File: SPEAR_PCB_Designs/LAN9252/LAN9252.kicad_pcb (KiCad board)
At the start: 2 copper layers, 68 parts, among them J1 SM04B-GHS-TB, J3 SM04B-GHS-TB, SW2 SW_MEC_5E, T1 H1102NLT, T2 H1102NLT, U1 LAN9252_ML, U2 24FC512, Y1 25MHz

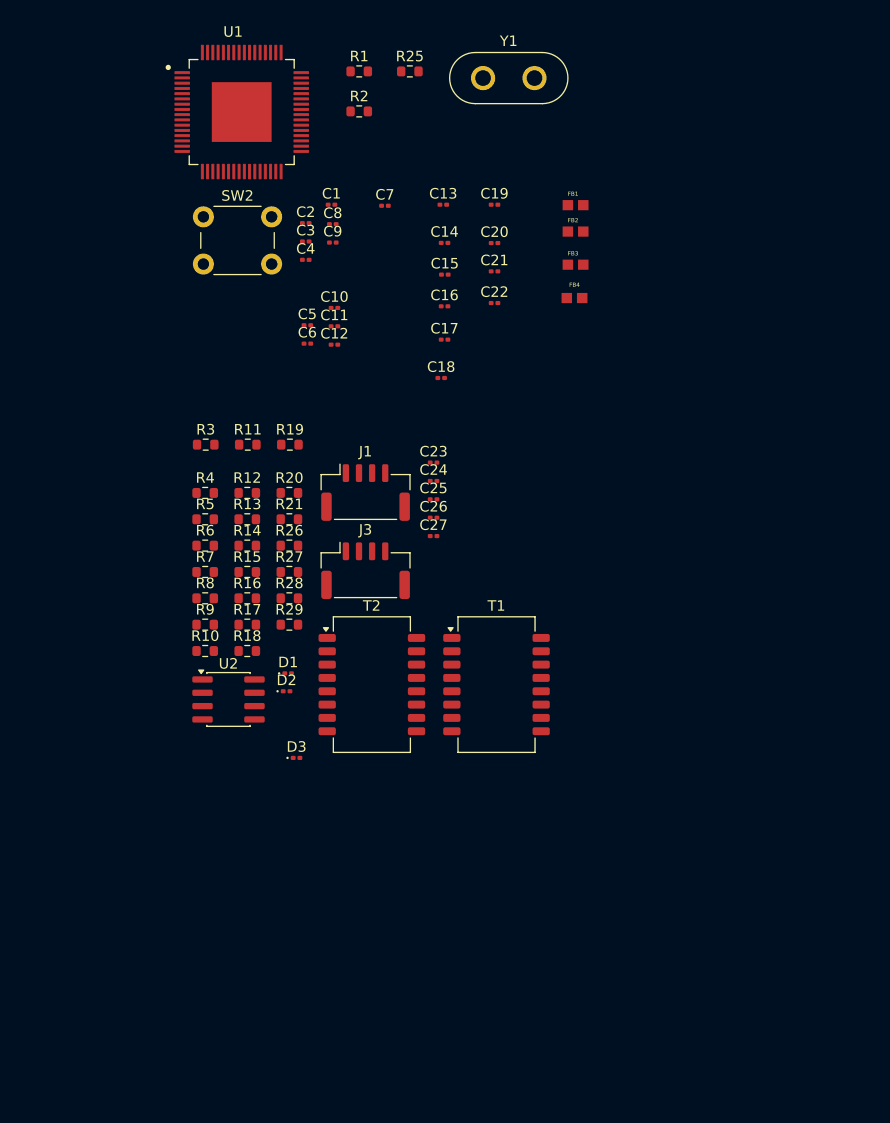
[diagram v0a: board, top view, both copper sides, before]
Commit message: Chris editted this.
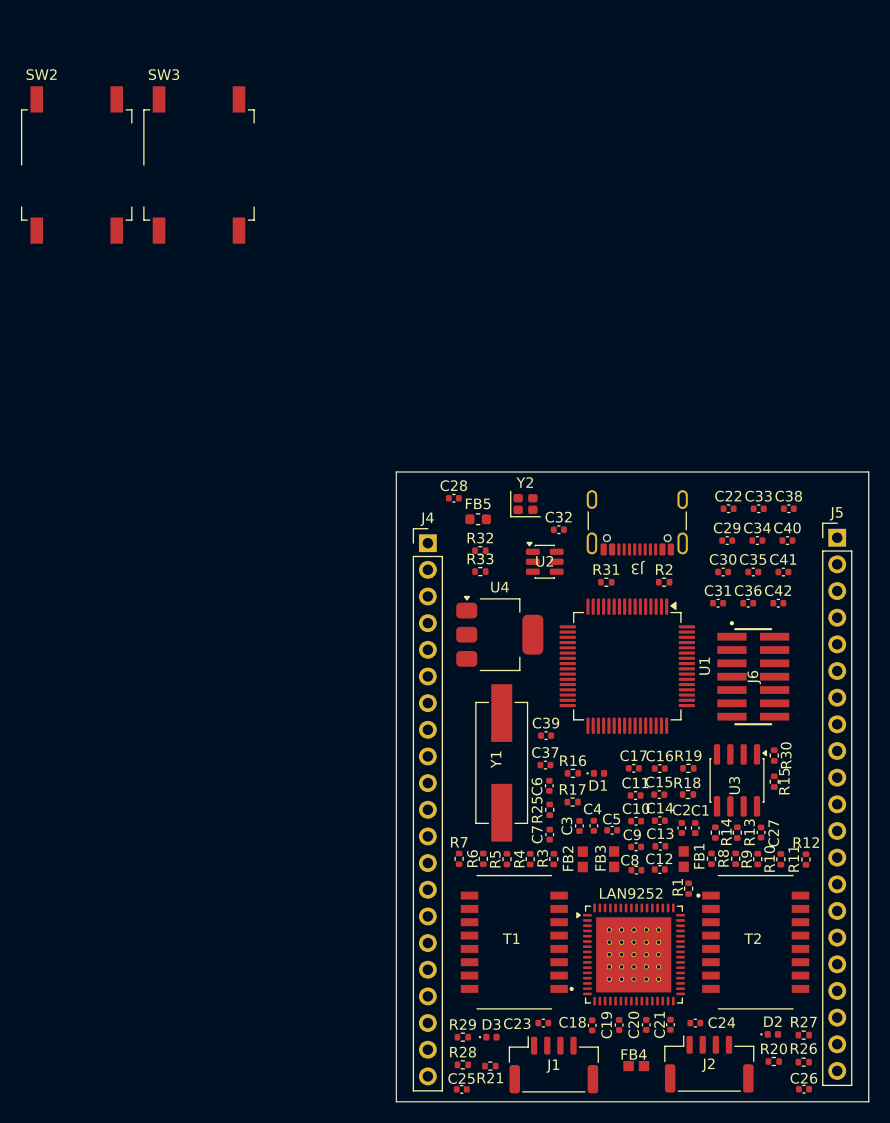
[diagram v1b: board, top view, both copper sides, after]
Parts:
- added C28: 10u, Capacitor_SMD:C_0402_1005Metric, F.Cu at (129.5, 90.8)
- added C29: 100n, Capacitor_SMD:C_0402_1005Metric, F.Cu at (155.5, 94.9)
- added C30: 10p, Capacitor_SMD:C_0402_1005Metric, F.Cu at (155.1, 97.9)
- added C31: 100n, Capacitor_SMD:C_0402_1005Metric, F.Cu at (154.7, 100.8)
- added C32: 100n, Capacitor_SMD:C_0402_1005Metric, F.Cu at (139.5, 93.8)
- added C33: 10p, Capacitor_SMD:C_0402_1005Metric, F.Cu at (158.5, 91.8)
- added C34: 100n, Capacitor_SMD:C_0402_1005Metric, F.Cu at (158.4, 94.9)
- added C35: 100n, Capacitor_SMD:C_0402_1005Metric, F.Cu at (158.0, 97.9)
- added C36: 2.2u, Capacitor_SMD:C_0402_1005Metric, F.Cu at (157.5, 100.8)
- added C37: 10u, Capacitor_SMD:C_0402_1005Metric, F.Cu at (138.2, 116.3)
- added C38: 100n, Capacitor_SMD:C_0402_1005Metric, F.Cu at (161.4, 91.8)
- added C39: 22u, Capacitor_SMD:C_0402_1005Metric, F.Cu at (138.3, 113.4)
- added C40: 10n, Capacitor_SMD:C_0402_1005Metric, F.Cu at (161.3, 94.9)
- added C41: 1u, Capacitor_SMD:C_0402_1005Metric, F.Cu at (160.9, 97.9)
- added C42: 1u, Capacitor_SMD:C_0402_1005Metric, F.Cu at (160.4, 100.8)
- added FB5: 120R, Inductor_SMD:L_0603_1608Metric, F.Cu at (131.8, 92.8)
- added J2: SM04B-GHS-TB, Connector_JST:JST_GH_SM04B-GHS-TB_1x04-1MP_P1.25mm_Horizontal, F.Cu at (153.8, 144.8)
- added J4: Conn_01x21_Pin, Connector_PinHeader_2.54mm:PinHeader_1x21_P2.54mm_Vertical, F.Cu at (127.0, 95.1)
- added J5: Conn_01x21_Pin, Connector_PinHeader_2.54mm:PinHeader_1x21_P2.54mm_Vertical, F.Cu at (166.0, 94.6)
- added J6: FTSH-107-01-F-DV-K-P-TR, SPEAR Footprints:SAMTEC_FTSH-107-01-F-DV-K-P-TR, F.Cu at (158.0, 107.8)
- added LAN9252: ~, SPEAR Footprints:LAN9252_QFN UPDATED, F.Cu at (146.6, 134.3)
- added R30: 100R, Resistor_SMD:R_0402_1005Metric, F.Cu at (160.0, 115.3)
- added R31: 5.1k, Resistor_SMD:R_0402_1005Metric, F.Cu at (144.0, 98.8)
- added R32: 5.1k, Resistor_SMD:R_0402_1005Metric, F.Cu at (132.0, 95.8)
- added R33: 5.1k, Resistor_SMD:R_0402_1005Metric, F.Cu at (132.0, 97.8)
- added SW3: SW_MEC_5E, Button_Switch_SMD:SW_MEC_5GSH9, F.Cu at (105.2, 59.1)
- added U3: 24FC512, Package_SO:SOIC-8_3.9x4.9mm_P1.27mm, F.Cu at (156.5, 117.7)
- added U4: AMS1117-3.3, Package_TO_SOT_SMD:SOT-223-3_TabPin2, F.Cu at (133.9, 103.8)
- added Y2: 16MHz, Crystal:Crystal_SMD_2016-4Pin_2.0x1.6mm, F.Cu at (136.3, 91.4)
- C1, C10, C11, C12, C13, C14, C15, C16, C17, C18, C19, C2, C20, C21, C23, C24, C25, C26, C27, C3, C4, C5, C6, C7, C8, C9: footprint Capacitor_SMD:C_0201_0603Metric -> Capacitor_SMD:C_0402_1005Metric
- C22: value 0.1uF -> 100n; footprint Capacitor_SMD:C_0201_0603Metric -> Capacitor_SMD:C_0402_1005Metric
- D1, D2, D3: footprint LED_SMD:LED_0201_0603Metric -> LED_SMD:LED_0402_1005Metric
- FB1, FB3, FB4: value BLM18EG221SN1D -> FerrriteBead; footprint Footprints SPEAR:Ferrite_bead -> SPEAR Footprints:Ferrite_bead
- FB2: value FerriteBead -> FerrriteBead; footprint Footprints SPEAR:Ferrite_bead -> SPEAR Footprints:Ferrite_bead
- J3: value SM04B-GHS-TB -> USB_C_Receptacle_USB2.0_16P; footprint Connector_JST:JST_GH_SM04B-GHS-TB_1x04-1MP_P1.25mm_Horizontal -> Connector_USB:USB_C_Receptacle_GCT_USB4105-xx-A_16P_TopMnt_Horizontal
- R1, R10, R11, R12, R13, R14, R15, R16, R17, R18, R19, R20, R21, R25, R26, R27, R28, R29, R3, R4, R5, R6, R7, R8, R9: footprint Resistor_SMD:R_0603_1608Metric -> Resistor_SMD:R_0402_1005Metric
- R2: value 10k -> 5.1k; footprint Resistor_SMD:R_0603_1608Metric -> Resistor_SMD:R_0402_1005Metric
- SW2: footprint Button_Switch_THT:SW_PUSH_6mm -> Button_Switch_SMD:SW_MEC_5GSH9
- T1, T2: footprint Transformer_SMD:Transformer_Pulse_H1100NL -> SPEAR Footprints:XFMR_H1102NLT
- U1: value LAN9252_ML -> STM32F446RCTx; footprint Footprints SPEAR:QFP50P1200X1200X120-65N -> Package_QFP:LQFP-64_10x10mm_P0.5mm
- U2: value 24FC512 -> USBLC6-2SC6; footprint Package_SO:SOIC-8_3.9x4.9mm_P1.27mm -> Package_TO_SOT_SMD:SOT-23-6
- Y1: footprint Crystal:Crystal_HC50_Vertical -> SPEAR Footprints:Y_Wurth_WE-XTAL_Quartz-HC49-4HSMX
- moved R1 83.9 mm to (151.8, 128.0), turned to -90 degrees
- moved C19 79.0 mm to (145.2, 141.0), turned to 90 degrees
- moved C20 75.9 mm to (147.8, 141.0), turned to 90 degrees
- moved C21 73.7 mm to (150.1, 141.0), turned to 90 degrees
- moved FB4 73.4 mm to (146.9, 144.9)
- moved R25 71.6 mm to (138.6, 120.5), turned to 90 degrees
- moved R20 71.2 mm to (160.0, 144.5)
- moved R26 69.4 mm to (162.8, 144.6), turned to 180 degrees
- moved C1 68.8 mm to (152.5, 122.3), turned to 90 degrees
- moved C8 68.0 mm to (146.9, 126.3)
- moved C2 67.9 mm to (151.2, 122.2), turned to 90 degrees
- moved R27 65.9 mm to (162.8, 142.0)
- moved Y1 65.3 mm to (134.0, 116.0), turned to 90 degrees
- moved C26 64.9 mm to (162.8, 147.1)
- moved C13 64.5 mm to (149.2, 124.0)
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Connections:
- C22 pad 1: /TP3 -> /EtherCAT/NRST
- C22 pad 2: GNDREF -> GND
- C7 pad 2: Net-(U1-OSCO) -> Net-(LAN9252-OSCO)
- D2 pad 1: Net-(D2-K) -> GND
- D2 pad 2: GND -> Net-(D2-A)
- D3 pad 1: Net-(D3-K) -> GND
- D3 pad 2: GND -> Net-(D3-A)
- FB3 pad 1: Net-(U1-VDD33BIAS) -> Net-(LAN9252-VDD33BIAS)
- R1 pad 2: Net-(U1-RBIAS) -> Net-(LAN9252-RBIAS)
- R15 pad 2: Net-(U2-A0) -> Net-(U3-A0)
- R2 pad 1: +3.3V -> Net-(J3-CC1)
- R2 pad 2: /TP3 -> GND
- R20 pad 2: Net-(D2-K) -> Net-(D2-A)
- R21 pad 2: Net-(D3-K) -> Net-(D3-A)
- R25 pad 2: Net-(U1-OSCI) -> Net-(LAN9252-OSCI)
- SW2 pad 1: GNDREF -> Net-(R33-Pad1)
- SW2 pad 2: GNDREF -> Net-(R33-Pad1)
- SW2 pad 3: /TP3 -> +3.3V
- SW2 pad 4: /TP3 -> +3.3V
- T1 pad 1: /TXB_P -> /TXA_P
- T1 pad 10: Net-(R27-Pad1) -> Net-(R29-Pad1)
- T1 pad 11: Net-(J3-Pin_3) -> Net-(J1-Pin_3)
- T1 pad 14: Net-(J3-Pin_2) -> Net-(J1-Pin_2)
- T1 pad 15: Net-(R26-Pad1) -> Net-(R28-Pad1)
- T1 pad 16: Net-(J3-Pin_1) -> Net-(J1-Pin_1)
- T1 pad 2: Net-(C24-Pad1) -> Net-(C23-Pad1)
- T1 pad 3: /TXB_N -> /TXA_N
- T1 pad 6: /RXB_P -> /RXA_P
- T1 pad 7: Net-(C24-Pad1) -> Net-(C23-Pad1)
- T1 pad 8: /RXB_N -> /RXA_N
- T1 pad 9: Net-(J3-Pin_4) -> Net-(J1-Pin_4)
- T2 pad 1: /TXA_P -> /TXB_P
- T2 pad 10: Net-(R29-Pad1) -> Net-(R27-Pad1)
- T2 pad 11: Net-(J1-Pin_3) -> Net-(J2-Pin_3)
- T2 pad 14: Net-(J1-Pin_2) -> Net-(J2-Pin_2)
- T2 pad 15: Net-(R28-Pad1) -> Net-(R26-Pad1)
- T2 pad 16: Net-(J1-Pin_1) -> Net-(J2-Pin_1)
- T2 pad 2: Net-(C23-Pad1) -> Net-(C24-Pad1)
- T2 pad 3: /TXA_N -> /TXB_N
- T2 pad 6: /RXA_P -> /RXB_P
- T2 pad 7: Net-(C23-Pad1) -> Net-(C24-Pad1)
- T2 pad 8: /RXA_N -> /RXB_N
- T2 pad 9: Net-(J1-Pin_4) -> Net-(J2-Pin_4)
- U1 pad 1: Net-(U1-OSCI) -> +3.3V
- U1 pad 10: unconnected-(U1-FXSDB/FXLOSB/~{FXSDENB}-Pad10) -> /EtherCAT/PC2
- U1 pad 11: unconnected-(U1-~{RST}-Pad11) -> /EtherCAT/PC3
- U1 pad 12: /D2/SIO2 -> GND
- U1 pad 13: /D1/SIO1 -> +3.3VA
- U1 pad 14: +3.3V -> /EtherCAT/PA0
- U1 pad 15: /D14/GPI8/GPO8/~{TX_SHIFT1} -> /EtherCAT/PA1
- U1 pad 16: /D13/GPI7/GPO7/~{TX_SHIFT0} -> /EtherCAT/PA2/UART2_TX
- U1 pad 17: /D0/SIO0 -> /EtherCAT/PA3/UART2_RX
- U1 pad 18: /SYNC1/LATCH1 -> GND
- U1 pad 19: /D9/LATCH_IN/SCK -> +3.3V
- U1 pad 2: Net-(U1-OSCO) -> /EtherCAT/PC13
- U1 pad 20: +3.3V -> /EtherCAT/PA4
- U1 pad 21: /D12/GPI6/GPO6 -> /SCK
- U1 pad 22: /D11/GPI5/GPO5 -> /MISO
- U1 pad 23: /D10/GPI4/GPO4 -> /MOSI
- U1 pad 24: /VDDCR -> /EtherCAT/PC4
- U1 pad 25: unconnected-(U1-A1/ALELO-Pad25) -> /EtherCAT/PC5
- U1 pad 26: unconnected-(U1-A3/GPI11/GPO11-Pad26) -> /EtherCAT/PB0
- U1 pad 27: unconnected-(U1-A4/GPI12/GPO12-Pad27) -> /EtherCAT/PB1
- U1 pad 28: /CS -> /EtherCAT/PB2
- U1 pad 29: unconnected-(U1-A2/ALEHI/GPI10/GPO10-Pad29) -> /EtherCAT/PB10
- U1 pad 3: unconnected-(U1-OSCVDD12-Pad3) -> /EtherCAT/PC14
- U1 pad 30: /WR/GPI14/GPO14 -> Net-(U1-VCAP_1)
- U1 pad 31: /RD/GPI15/GPO15 -> GND
- U1 pad 33: /A0/D15/GPI9/GPO9 -> /EtherCAT/PB12
- U1 pad 34: /SYNC0/LATCH0 -> /EtherCAT/PB13
- U1 pad 35: /D3/SIO3 -> /EtherCAT/PB14
- U1 pad 36: /D6/GPI0/GPO0 -> /EtherCAT/PB15
- U1 pad 37: +3.3V -> /EtherCAT/PC6
- U1 pad 38: /VDDCR -> /EtherCAT/PC7
- U1 pad 39: /D7/GPI1/GPO1 -> /EtherCAT/PC8
- U1 pad 4: GNDREF -> /EtherCAT/PC15
- U1 pad 40: /D8/GPI2/GPO2 -> /EtherCAT/PC9
- U1 pad 41: GNDREF -> /EtherCAT/PA8
- U1 pad 42: /I2C_SDL -> /EtherCAT/PA9
- U1 pad 43: /I2C_SCL -> /EtherCAT/PA10
- U1 pad 44: /IRQ -> /EtherCAT/USB_D-
- U1 pad 45: /GPIO2 -> /EtherCAT/USB_D+
- U1 pad 46: /GPIO1 -> /EtherCAT/SWDIO
- U1 pad 47: +3.3V -> GND
- U1 pad 48: /GPIO0 -> +3.3V
- U1 pad 49: /D4/GPI3/GPO3 -> /EtherCAT/SWCLK
- U1 pad 5: +3.3V -> /EtherCAT/HSE_IN
- U1 pad 50: /D5/OUTVALID/~{SCS} -> /EtherCAT/PA15
- U1 pad 51: /VDD33TXRX1 -> /EtherCAT/PC10
- U1 pad 52: /TXA_N -> /EtherCAT/PC11
- U1 pad 53: /TXA_P -> /EtherCAT/PC12
- U1 pad 54: /RXA_N -> unconnected-(U1-PD2-Pad54)
- U1 pad 55: /RXA_P -> /EtherCAT/SWO
- U1 pad 56: /VDD12TX1 -> /EtherCAT/PB4
- U1 pad 57: Net-(U1-RBIAS) -> /EtherCAT/PB5
- U1 pad 58: Net-(U1-VDD33BIAS) -> /EtherCAT/PB6
- U1 pad 59: /VDD12TX1 -> /EtherCAT/PB7
- U1 pad 6: /VDDCR -> /EtherCAT/HSE_OUT
- U1 pad 60: /RXB_P -> /EtherCAT/BOOT0
- U1 pad 61: /RXB_N -> /EtherCAT/PB8
- U1 pad 62: /TXB_P -> /EtherCAT/PB9
- U1 pad 63: /TXB_N -> GND
- U1 pad 64: /VDD33TXRX2 -> +3.3V
- U1 pad 7: +3.3V -> /EtherCAT/NRST
- U1 pad 8: GNDREF -> /EtherCAT/PC0
- U1 pad 9: GNDREF -> /EtherCAT/PC1
- U2 pad 1: Net-(U2-A0) -> Net-(J3-D--PadA7)
- U2 pad 2: Net-(U2-A0) -> GND
- U2 pad 3: Net-(U2-A0) -> Net-(J3-D+-PadA6)
- U2 pad 4: GNDREF -> /EtherCAT/USB_D+
- U2 pad 5: /I2C_SDL -> +VBUS
- U2 pad 6: /I2C_SCL -> /EtherCAT/USB_D-
- Y1 pad 1: Net-(U1-OSCO) -> Net-(LAN9252-OSCO)
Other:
- board outline added: 45 x 60 mm

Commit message: changes to lan setting
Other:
- copper layers 2 -> 4
- rule pad_to_mask_clearance: 0 -> 0.1
